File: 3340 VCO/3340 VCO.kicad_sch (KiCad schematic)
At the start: 74 parts, among them J1 Conn_02x05_Odd_Even, J2 Conn_01x19, U1 TL072, U2 TL072, U3 TL072, U4 AS3340, U6 LM7905_TO220

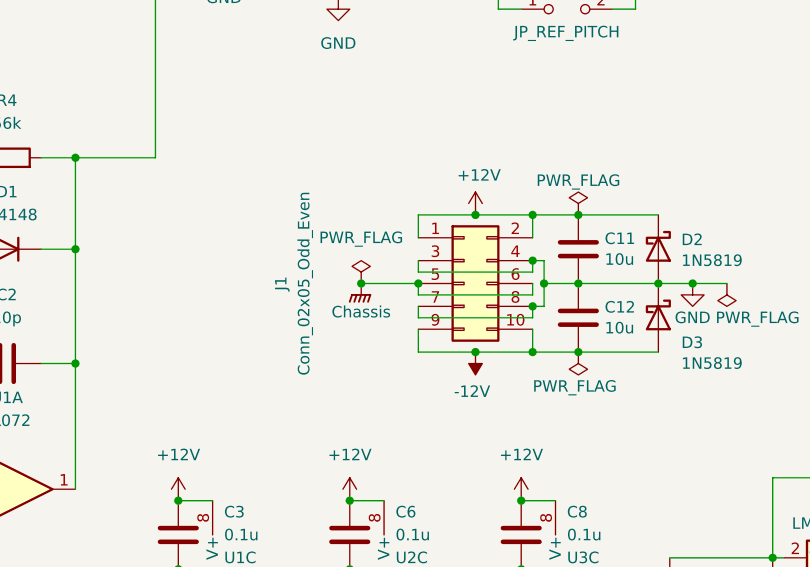
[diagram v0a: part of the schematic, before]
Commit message: Finish VCO
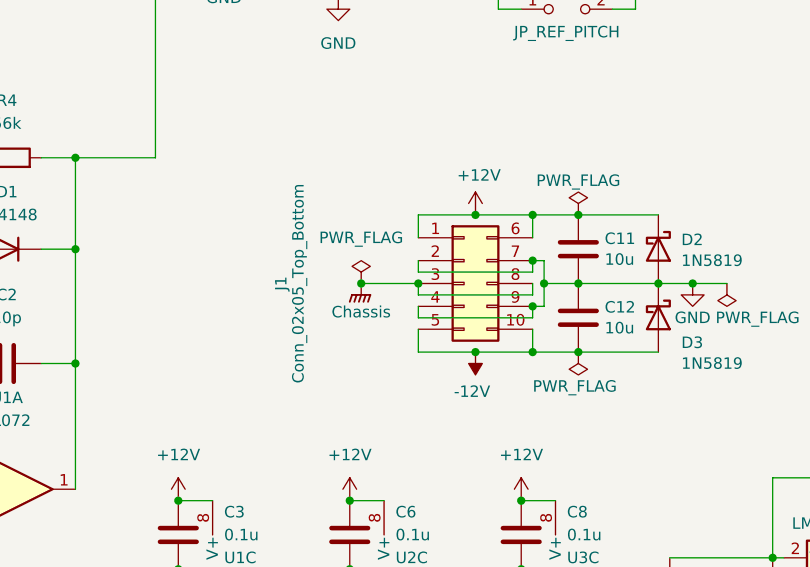
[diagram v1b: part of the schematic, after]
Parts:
- J1: value Conn_02x05_Odd_Even -> Conn_02x05_Top_Bottom; symbol Connector_Generic:Conn_02x05_Odd_Even -> Connector_Generic:Conn_02x05_Top_Bottom
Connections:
- net +12V: now also J1.6 (Pin_6); no longer J1.2 (Pin_2)
- net -12V: now also J1.5 (Pin_5); no longer J1.9 (Pin_9)
- net Chassis: now also J1.3 (Pin_3), J1.8 (Pin_8); no longer J1.5 (Pin_5), J1.6 (Pin_6)
- net GND: now also J1.2 (Pin_2), J1.9 (Pin_9); no longer J1.3 (Pin_3), J1.8 (Pin_8)
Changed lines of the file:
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@@
     )
   )
-  (symbol (lib_id "Connector_Generic:Conn_02x05_Odd_Even") (at 105.41 146.05 0) (unit 1)
+  (symbol (lib_id "Connector_Generic:Conn_02x05_Top_Bottom") (at 105.41 146.05 0) (unit 1)
     (in_bom yes) (on_board yes) (dnp no)
     (property "Reference" "J1" (at 85.09 146.05 90)
       (effects (font (size 1.27 1.27)))
     )
-    (property "Value" "Conn_02x05_Odd_Even" (at 87.63 146.05 90)
+    (property "Value" "Conn_02x05_Top_Bottom" (at 86.995 146.05 90)
       (effects (font (size 1.27 1.27)))
     )
